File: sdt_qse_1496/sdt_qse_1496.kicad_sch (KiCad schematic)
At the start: 93 parts, among them J1 Conn_02x08_Odd_Even, J2 SJ-3524-SMT, J3 5-1814832-1, J4 5-1814832-1, J6 Conn_01x02_Male, Q1 Q_NPN_BEC, Q2 Q_NPN_BEC, Q3 Q_PMOS_GSD, Q4 Q_PMOS_GSD, U1 SN74AC74PW, U2 MC1496DR2G, U3 Toroidal_Transformer, U4 MC1496DR2G

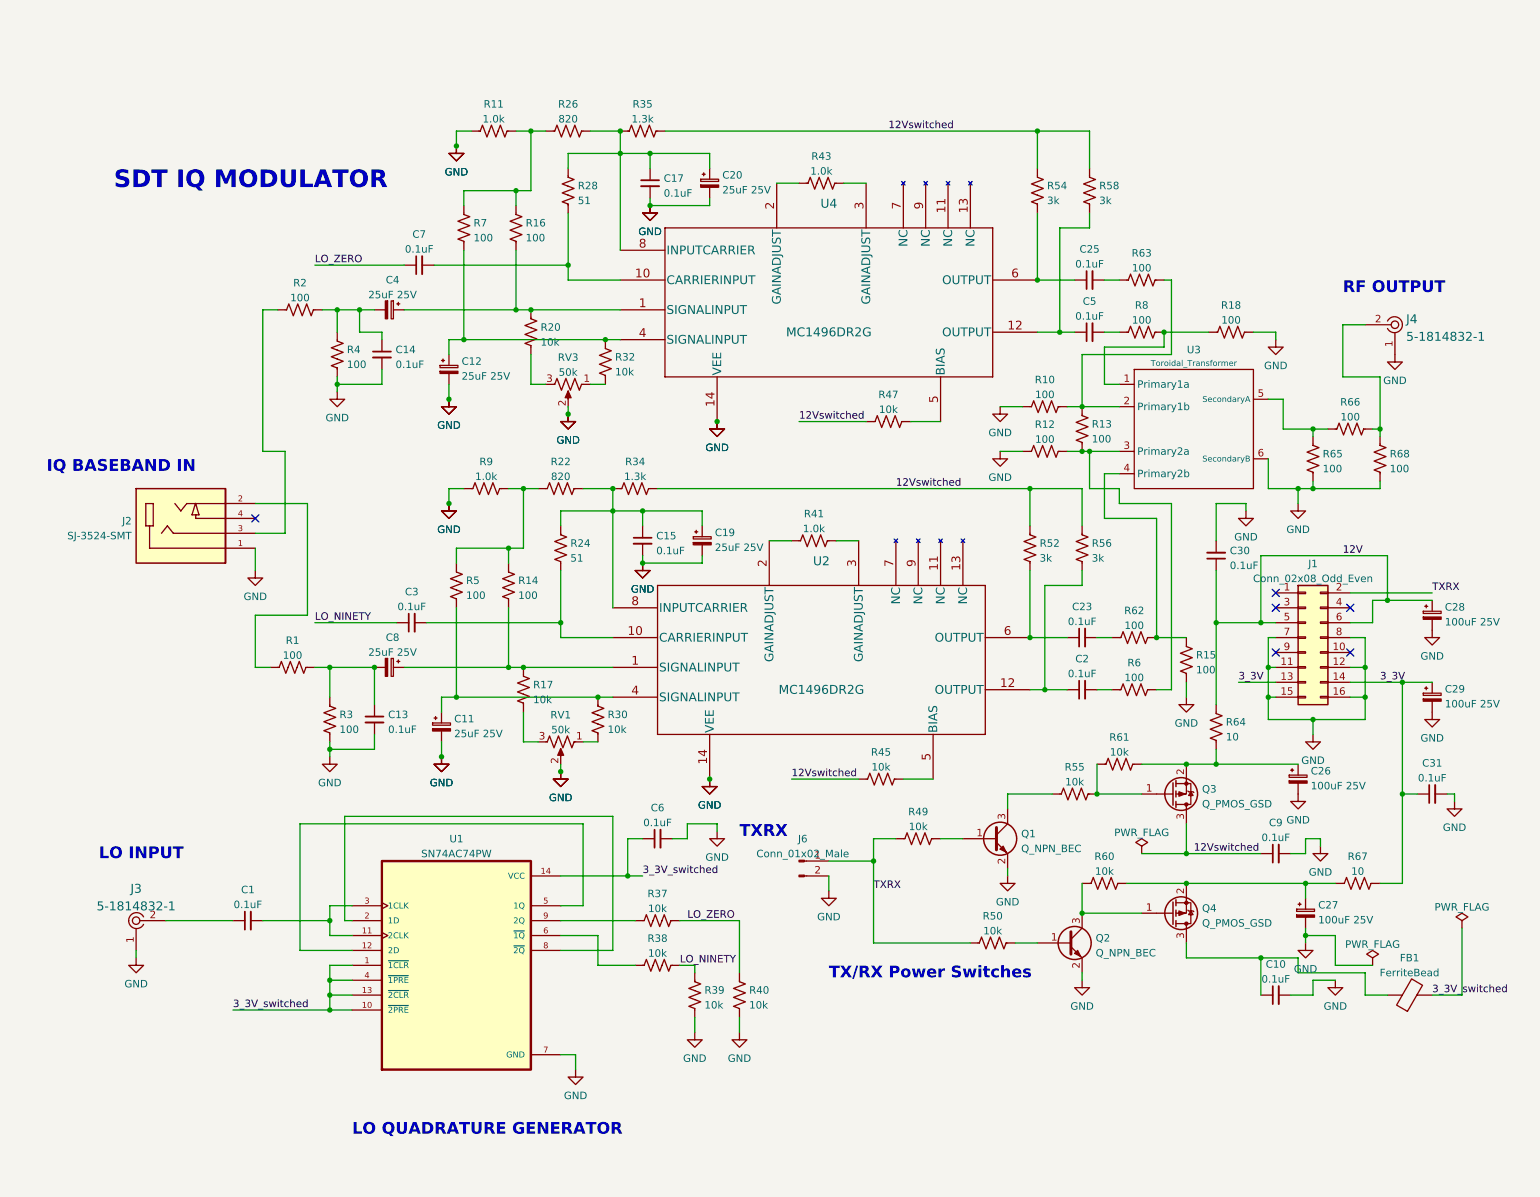
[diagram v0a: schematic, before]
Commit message: More simulations working.
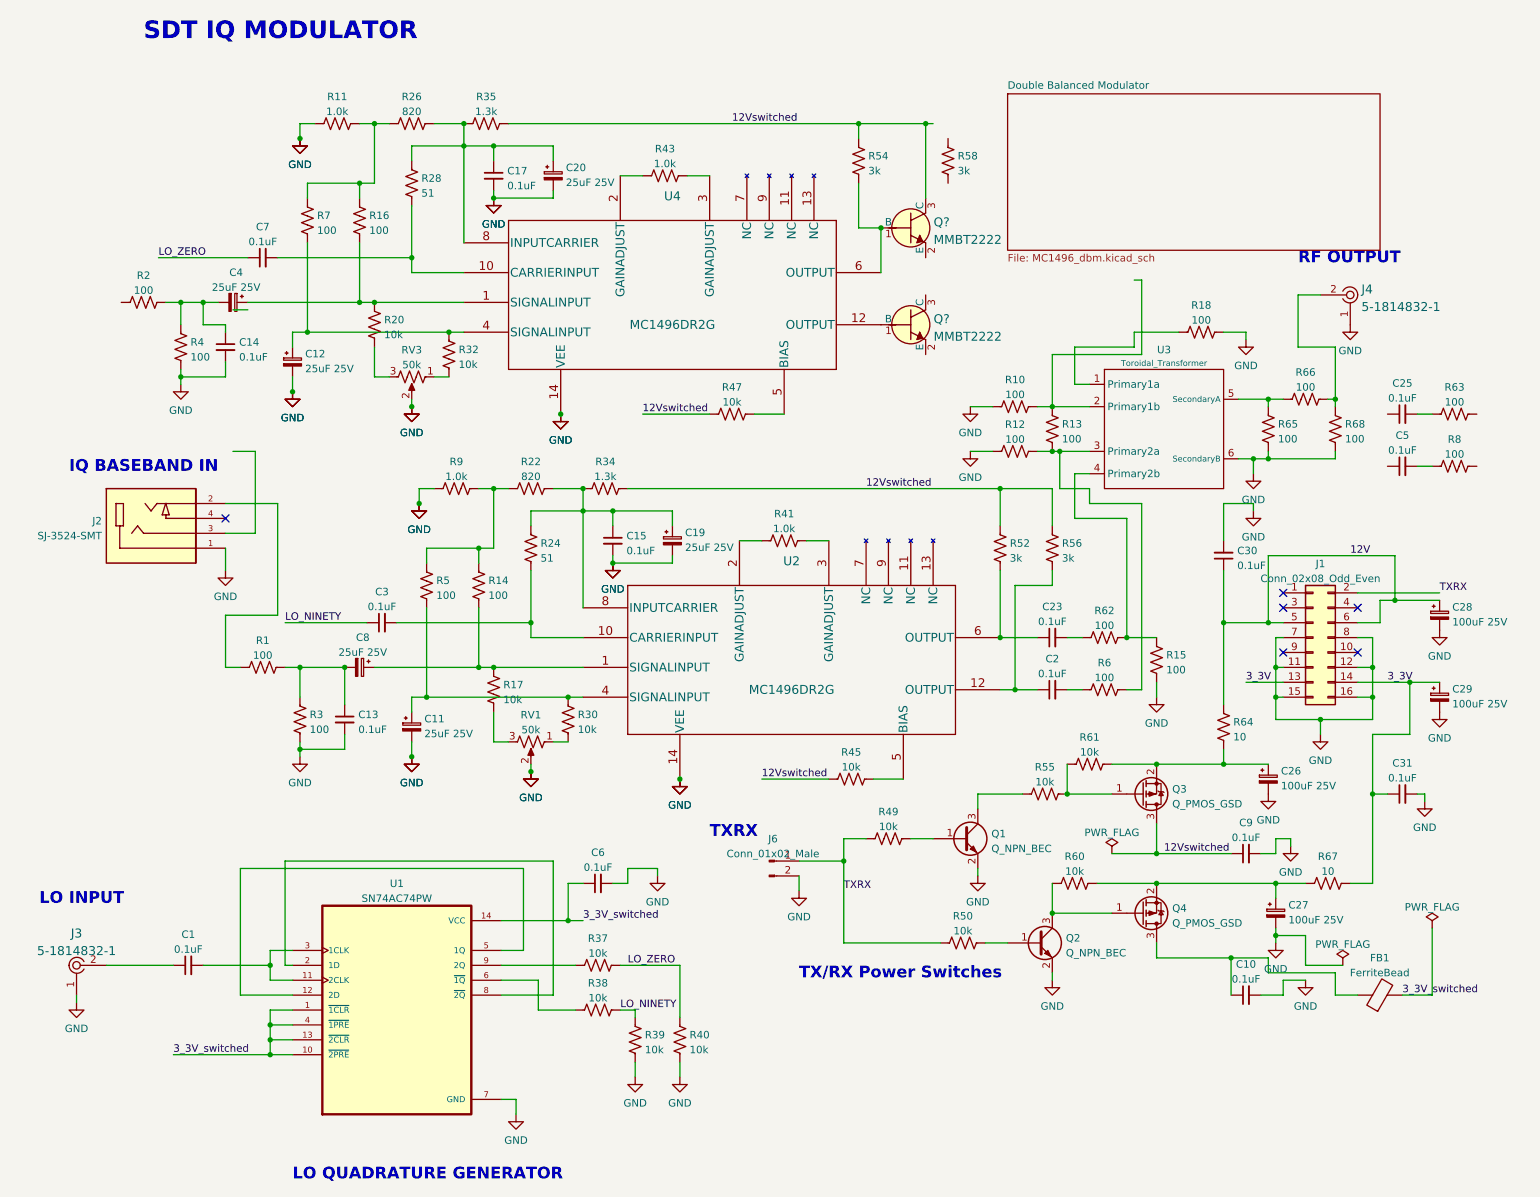
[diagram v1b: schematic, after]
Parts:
- added Q? (x2): MMBT2222, digikey-footprints:SOT-23-3, symbol dk_Transistors-Bipolar-BJT-Single:MMBT2222LT1G
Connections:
- net 12Vswitched: now also Q?.3 (C); no longer R58.1
- net at R10.2, R13.2, U3.2 (Primary1b): no longer R63.2
- net at R2.1: no longer J2.3
- net at R18.1, U3.1 (Primary1a): no longer R8.2
- net at R54.2, U4.6 (OUTPUT): now also Q?.1 (B); no longer C25.1
- new net: Q?.1 (B), U4.12 (OUTPUT)
- now unconnected: C5.1, R58.2
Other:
- added sheet Double Balanced Modulator (MC1496_dbm.kicad_sch)
- moved on the sheet: C1, C10, C11, C12, C13, C14, C15, C17, C19, C2, C20, C23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
